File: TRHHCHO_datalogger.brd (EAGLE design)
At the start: 49.1 x 50.8 mm, 39 parts, among them J6 AMP FCI 10103594-0001LF, U1 ATMEGA328P-MU, U10 TSL2591, U2 FT231XQ-R, U3 DS3234, U7 SHT31/35, U8 MCP1703/3.3V, Y2 SPARKFUN_RESONATORSMD

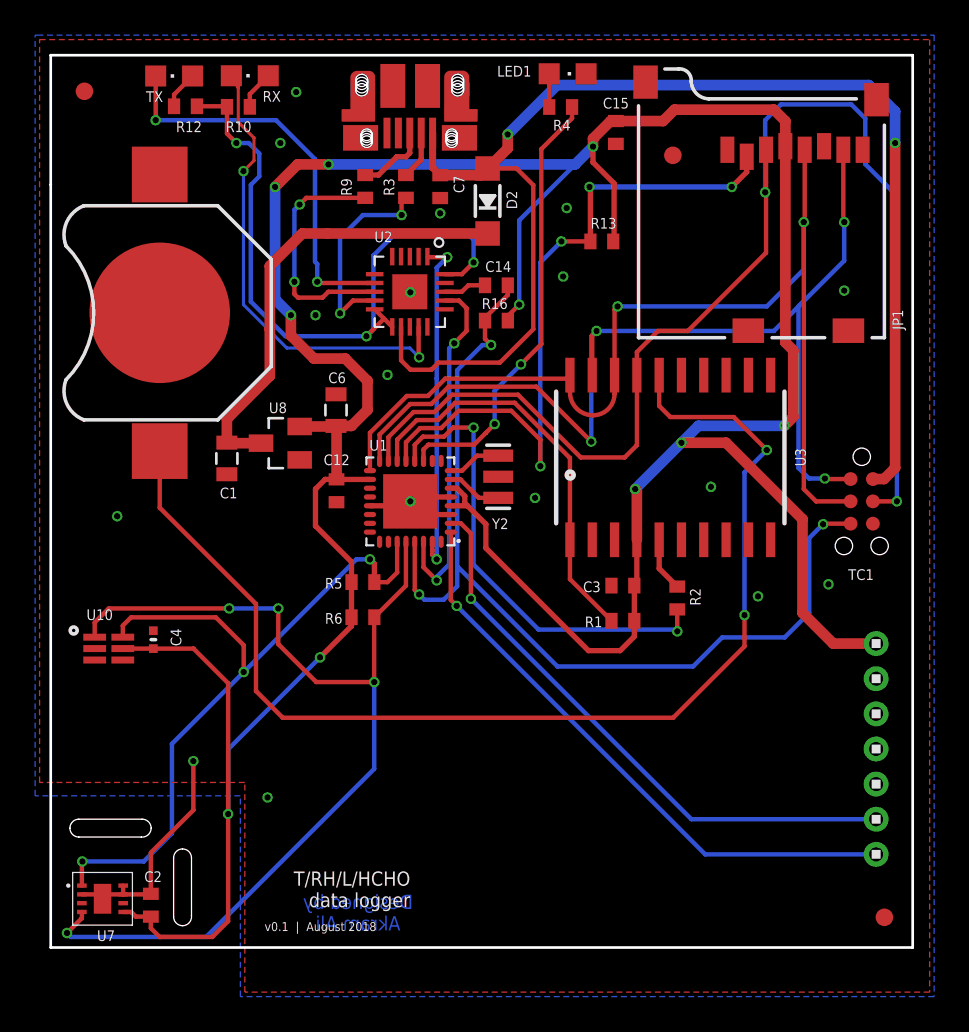
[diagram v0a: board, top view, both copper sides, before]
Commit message: Revert "update"
This reverts commit 3fd739265b7c9a937414b5746fef9af12a5aee94.
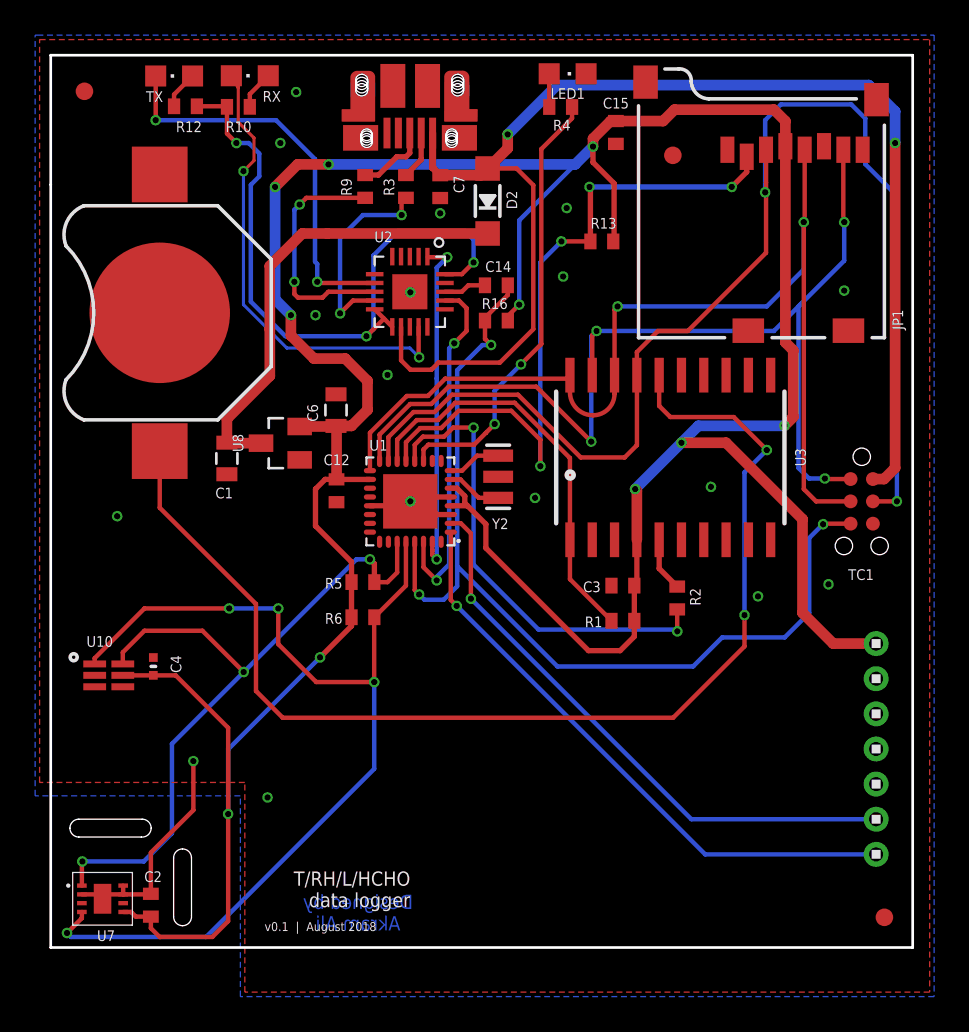
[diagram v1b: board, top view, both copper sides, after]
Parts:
- moved C4 1.52 mm to (14.0, 16.0)
- moved U10 1.52 mm to (11.4, 15.5)
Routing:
- net VCC: track 197.5 -> 195.4 mm
- net SDA: track 42.5 -> 41.6 mm
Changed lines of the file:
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@@
 <element name="LED1" library="adafruit" package="CHIPLED_0805" value="Blue" x="37.5562" y="49.7432" smashed="yes" rot="R270">
 <attribute name="MPN" value="150080BS75000" x="37.5562" y="49.7432" size="1.778" layer="27" rot="R270" display="off"/>
-<attribute name="NAME" x="33.5382" y="49.5832" size="0.6096" layer="25" font="vector"/>
+<attribute name="NAME" x="36.5862" y="48.3132" size="0.6096" layer="25" font="vector"/>
 </element>
 <element name="U8" library="linear" library_urn="urn:adsk.eagle:library:262" package="SOT23" value="MCP1703/3.3V" x="21.1992" y="28.7124" smashed="yes" rot="R90">
 <attribute name="MPN" value="MCP1703T-2502E/CB" x="21.1992" y="28.7124" size="1.778" layer="27" rot="R90" display="off"/>
-<attribute name="NAME" x="21.5766" y="31.0322" size="0.6096" layer="25" font="vector" rot="R180"/>
+<attribute name="NAME" x="19.0942" y="28.2074" size="0.6096" layer="25" font="vector" rot="R90"/>
 </element>
 <element name="C1" library="SparkFun-Capacitors" package="0805" value="1uF" x="18.1558" y="27.8426" smashed="yes" rot="R270">
 <attribute name="MPN" value="CC0805KKX7R7BB105" x="18.1558" y="27.8426" size="1.778" layer="27" rot="R270" display="off"/>
-<attribute name="NAME" x="17.7524" y="25.5703" size="0.6096" layer="25" font="vector"/>
+<attribute name="NAME" x="17.4984" y="25.5703" size="0.6096" layer="25" font="vector"/>
 </element>
 <element name="C6" library="SparkFun-Capacitors" package="0805" value="1uF" x="24.3674" y="30.5942" smashed="yes" rot="R90">
 <attribute name="MPN" value="CC0805KKX7R7BB105" x="24.3674" y="30.5942" size="1.778" layer="27" rot="R90" display="off"/>
-<attribute name="NAME" x="24.9318" y="32.7399" size="0.6096" layer="25" font="vector" rot="R180"/>
+<attribute name="NAME" x="23.3419" y="29.9322" size="0.6096" layer="25" font="vector" rot="R90"/>
 </element>
 <element name="RX" library="adafruit" package="CHIPLED_0805" value="Yellow" x="19.4596" y="49.6314" smashed="yes" rot="R90">
@@
 </element>
 <element name="U$4" library="headers(2mm)" package="1X7" value="1X7" x="55.118" y="11.303" rot="R90"/>
-<element name="U10" library="TSL2591" package="DFN6_TAOS" value="TSL2591" x="11.43" y="17.018" smashed="yes">
-<attribute name="MPN" value="TSL25911FN " x="11.43" y="17.018" size="1.778" layer="27" display="off"/>
-<attribute name="NAME" x="10.16" y="18.642" size="0.6096" layer="25" font="vector"/>
-</element>
-<element name="C4" library="Adafruit Feather 32u4 Bluefruit LE" package="MICROBUILDER__0402MP" value="0.1uF" x="13.97" y="17.526" smashed="yes" rot="R270">
-<attribute name="MPN" value="GRM155R71C104KA88J" x="13.97" y="17.526" size="1.778" layer="27" rot="R270" display="off"/>
-<attribute name="NAME" x="14.9543" y="18.161" size="0.6096" layer="25" font="vector" rot="R270"/>
+<element name="U10" library="TSL2591" package="DFN6_TAOS" value="TSL2591" x="11.43" y="15.494" smashed="yes">
+<attribute name="MPN" value="TSL25911FN " x="11.43" y="15.494" size="1.778" layer="27" display="off"/>
+<attribute name="NAME" x="10.16" y="17.118" size="0.6096" layer="25" font="vector"/>
+</element>
+<element name="C4" library="Adafruit Feather 32u4 Bluefruit LE" package="MICROBUILDER__0402MP" value="0.1uF" x="13.97" y="16.002" smashed="yes" rot="R270">
+<attribute name="MPN" value="GRM155R71C104KA88J" x="13.97" y="16.002" size="1.778" layer="27" rot="R270" display="off"/>
+<attribute name="NAME" x="14.9543" y="16.637" size="0.6096" layer="25" font="vector" rot="R270"/>
 </element>
 </elements>
@@
 <contactref element="C4" pad="2"/>
 <contactref element="U10" pad="5"/>
-<wire x1="12.23" y1="17.018" x2="13.97" y2="17.018" width="0.254" layer="1"/>
-<wire x1="18.228" y1="15.046" x2="16.256" y2="17.018" width="0.254" layer="1"/>
-<wire x1="18.228" y1="7.6" x2="18.228" y2="15.046" width="0.254" layer="1"/>
+<wire x1="12.23" y1="15.494" x2="13.97" y2="15.494" width="0.254" layer="1"/>
+<wire x1="13.97" y1="15.494" x2="15.24" y2="15.494" width="0.254" layer="1"/>
+<wire x1="18.228" y1="12.506" x2="15.24" y2="15.494" width="0.254" layer="1"/>
+<wire x1="18.228" y1="7.6" x2="18.228" y2="12.506" width="0.254" layer="1"/>
 <wire x1="25.252" y1="18.308" x2="25.252" y2="18.8032" width="0.3048" layer="1"/>
-<wire x1="16.256" y1="17.018" x2="13.97" y2="17.018" width="0.254" layer="1"/>
 </signal>
 <signal name="SCL">
@@
 <wire x1="26.543" y1="18.7942" x2="26.552" y2="18.8032" width="0.254" layer="1"/>
 <contactref element="U10" pad="1"/>
-<wire x1="10.63" y1="17.668" x2="10.63" y2="18.504" width="0.254" layer="1"/>
-<wire x1="10.63" y1="18.504" x2="11.43" y2="19.304" width="0.254" layer="1"/>
-<wire x1="11.43" y1="19.304" x2="18.288" y2="19.304" width="0.254" layer="1"/>
+<wire x1="10.63" y1="16.144" x2="10.63" y2="16.472" width="0.254" layer="1"/>
+<wire x1="10.63" y1="16.472" x2="13.462" y2="19.304" width="0.254" layer="1"/>
+<wire x1="13.462" y1="19.304" x2="18.288" y2="19.304" width="0.254" layer="1"/>
 <via x="18.288" y="19.304" extent="1-16" drill="0.35"/>
 <wire x1="18.288" y1="19.304" x2="21.082" y2="19.304" width="0.254" layer="16"/>
@@
 <contactref element="U10" pad="6"/>
 <wire x1="19.1135" y1="15.6845" x2="15.028" y2="11.599" width="0.254" layer="16"/>
-<wire x1="12.23" y1="17.668" x2="12.23" y2="18.326" width="0.254" layer="1"/>
-<wire x1="12.23" y1="18.326" x2="12.7" y2="18.796" width="0.254" layer="1"/>
-<wire x1="12.7" y1="18.796" x2="17.526" y2="18.796" width="0.254" layer="1"/>
-<wire x1="17.526" y1="18.796" x2="19.1135" y2="17.2085" width="0.254" layer="1"/>
+<wire x1="12.23" y1="16.144" x2="12.23" y2="16.802" width="0.254" layer="1"/>
+<wire x1="12.23" y1="16.802" x2="13.462" y2="18.034" width="0.254" layer="1"/>
+<wire x1="13.462" y1="18.034" x2="16.764" y2="18.034" width="0.254" layer="1"/>
+<wire x1="16.764" y1="18.034" x2="19.1135" y2="15.6845" width="0.254" layer="1"/>
 <via x="19.1135" y="15.6845" extent="1-16" drill="0.35"/>
-<wire x1="19.1135" y1="17.2085" x2="19.1135" y2="15.6845" width="0.254" layer="1"/>
 </signal>
 <signal name="N$4">

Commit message: update
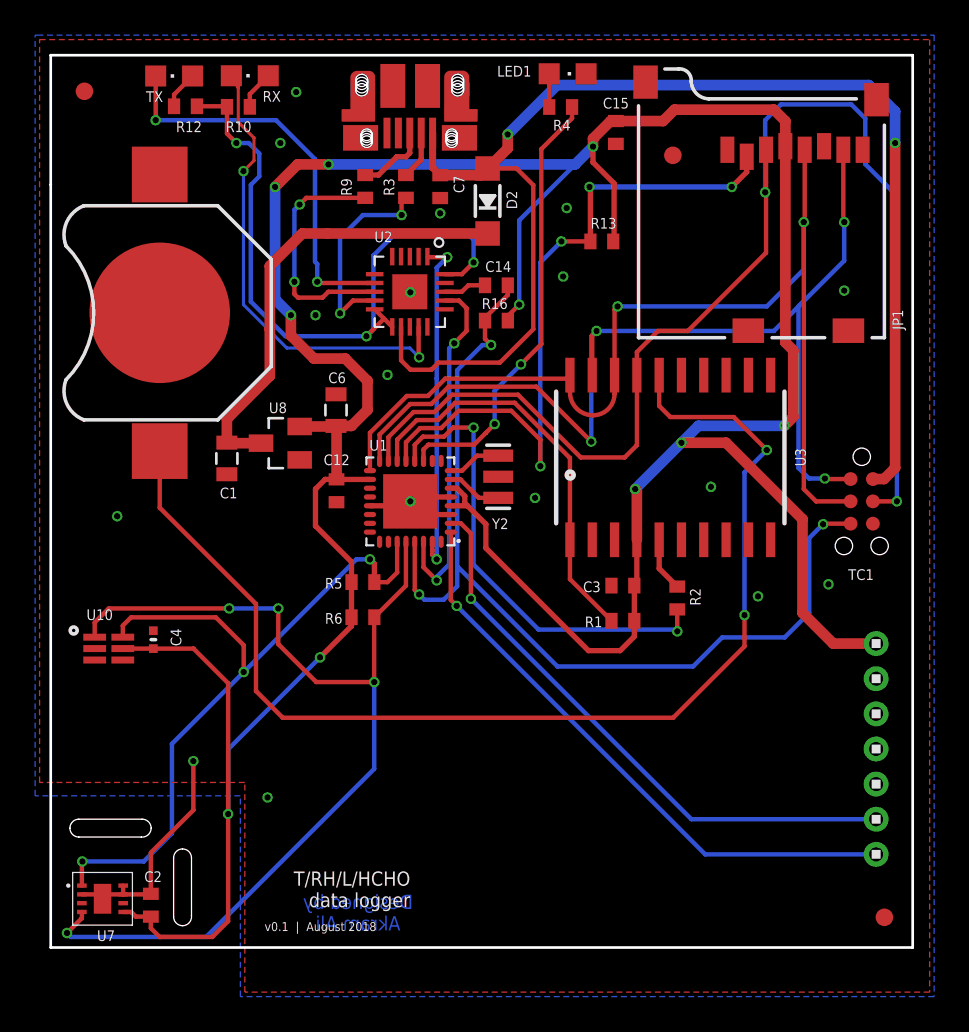
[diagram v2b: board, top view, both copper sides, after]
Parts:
- moved C4 1.52 mm to (14.0, 17.5)
- moved U10 1.52 mm to (11.4, 17.0)
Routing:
- net VCC: track 195.4 -> 197.5 mm
- net SDA: track 41.6 -> 42.5 mm
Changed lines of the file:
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@@
 <element name="LED1" library="adafruit" package="CHIPLED_0805" value="Blue" x="37.5562" y="49.7432" smashed="yes" rot="R270">
 <attribute name="MPN" value="150080BS75000" x="37.5562" y="49.7432" size="1.778" layer="27" rot="R270" display="off"/>
-<attribute name="NAME" x="36.5862" y="48.3132" size="0.6096" layer="25" font="vector"/>
+<attribute name="NAME" x="33.5382" y="49.5832" size="0.6096" layer="25" font="vector"/>
 </element>
 <element name="U8" library="linear" library_urn="urn:adsk.eagle:library:262" package="SOT23" value="MCP1703/3.3V" x="21.1992" y="28.7124" smashed="yes" rot="R90">
 <attribute name="MPN" value="MCP1703T-2502E/CB" x="21.1992" y="28.7124" size="1.778" layer="27" rot="R90" display="off"/>
-<attribute name="NAME" x="19.0942" y="28.2074" size="0.6096" layer="25" font="vector" rot="R90"/>
+<attribute name="NAME" x="21.5766" y="31.0322" size="0.6096" layer="25" font="vector" rot="R180"/>
 </element>
 <element name="C1" library="SparkFun-Capacitors" package="0805" value="1uF" x="18.1558" y="27.8426" smashed="yes" rot="R270">
 <attribute name="MPN" value="CC0805KKX7R7BB105" x="18.1558" y="27.8426" size="1.778" layer="27" rot="R270" display="off"/>
-<attribute name="NAME" x="17.4984" y="25.5703" size="0.6096" layer="25" font="vector"/>
+<attribute name="NAME" x="17.7524" y="25.5703" size="0.6096" layer="25" font="vector"/>
 </element>
 <element name="C6" library="SparkFun-Capacitors" package="0805" value="1uF" x="24.3674" y="30.5942" smashed="yes" rot="R90">
 <attribute name="MPN" value="CC0805KKX7R7BB105" x="24.3674" y="30.5942" size="1.778" layer="27" rot="R90" display="off"/>
-<attribute name="NAME" x="23.3419" y="29.9322" size="0.6096" layer="25" font="vector" rot="R90"/>
+<attribute name="NAME" x="24.9318" y="32.7399" size="0.6096" layer="25" font="vector" rot="R180"/>
 </element>
 <element name="RX" library="adafruit" package="CHIPLED_0805" value="Yellow" x="19.4596" y="49.6314" smashed="yes" rot="R90">
@@
 </element>
 <element name="U$4" library="headers(2mm)" package="1X7" value="1X7" x="55.118" y="11.303" rot="R90"/>
-<element name="U10" library="TSL2591" package="DFN6_TAOS" value="TSL2591" x="11.43" y="15.494" smashed="yes">
-<attribute name="MPN" value="TSL25911FN " x="11.43" y="15.494" size="1.778" layer="27" display="off"/>
-<attribute name="NAME" x="10.16" y="17.118" size="0.6096" layer="25" font="vector"/>
-</element>
-<element name="C4" library="Adafruit Feather 32u4 Bluefruit LE" package="MICROBUILDER__0402MP" value="0.1uF" x="13.97" y="16.002" smashed="yes" rot="R270">
-<attribute name="MPN" value="GRM155R71C104KA88J" x="13.97" y="16.002" size="1.778" layer="27" rot="R270" display="off"/>
-<attribute name="NAME" x="14.9543" y="16.637" size="0.6096" layer="25" font="vector" rot="R270"/>
+<element name="U10" library="TSL2591" package="DFN6_TAOS" value="TSL2591" x="11.43" y="17.018" smashed="yes">
+<attribute name="MPN" value="TSL25911FN " x="11.43" y="17.018" size="1.778" layer="27" display="off"/>
+<attribute name="NAME" x="10.16" y="18.642" size="0.6096" layer="25" font="vector"/>
+</element>
+<element name="C4" library="Adafruit Feather 32u4 Bluefruit LE" package="MICROBUILDER__0402MP" value="0.1uF" x="13.97" y="17.526" smashed="yes" rot="R270">
+<attribute name="MPN" value="GRM155R71C104KA88J" x="13.97" y="17.526" size="1.778" layer="27" rot="R270" display="off"/>
+<attribute name="NAME" x="14.9543" y="18.161" size="0.6096" layer="25" font="vector" rot="R270"/>
 </element>
 </elements>
@@
 <contactref element="C4" pad="2"/>
 <contactref element="U10" pad="5"/>
-<wire x1="12.23" y1="15.494" x2="13.97" y2="15.494" width="0.254" layer="1"/>
-<wire x1="13.97" y1="15.494" x2="15.24" y2="15.494" width="0.254" layer="1"/>
-<wire x1="18.228" y1="12.506" x2="15.24" y2="15.494" width="0.254" layer="1"/>
-<wire x1="18.228" y1="7.6" x2="18.228" y2="12.506" width="0.254" layer="1"/>
+<wire x1="12.23" y1="17.018" x2="13.97" y2="17.018" width="0.254" layer="1"/>
+<wire x1="18.228" y1="15.046" x2="16.256" y2="17.018" width="0.254" layer="1"/>
+<wire x1="18.228" y1="7.6" x2="18.228" y2="15.046" width="0.254" layer="1"/>
 <wire x1="25.252" y1="18.308" x2="25.252" y2="18.8032" width="0.3048" layer="1"/>
+<wire x1="16.256" y1="17.018" x2="13.97" y2="17.018" width="0.254" layer="1"/>
 </signal>
 <signal name="SCL">
@@
 <wire x1="26.543" y1="18.7942" x2="26.552" y2="18.8032" width="0.254" layer="1"/>
 <contactref element="U10" pad="1"/>
-<wire x1="10.63" y1="16.144" x2="10.63" y2="16.472" width="0.254" layer="1"/>
-<wire x1="10.63" y1="16.472" x2="13.462" y2="19.304" width="0.254" layer="1"/>
-<wire x1="13.462" y1="19.304" x2="18.288" y2="19.304" width="0.254" layer="1"/>
+<wire x1="10.63" y1="17.668" x2="10.63" y2="18.504" width="0.254" layer="1"/>
+<wire x1="10.63" y1="18.504" x2="11.43" y2="19.304" width="0.254" layer="1"/>
+<wire x1="11.43" y1="19.304" x2="18.288" y2="19.304" width="0.254" layer="1"/>
 <via x="18.288" y="19.304" extent="1-16" drill="0.35"/>
 <wire x1="18.288" y1="19.304" x2="21.082" y2="19.304" width="0.254" layer="16"/>
@@
 <contactref element="U10" pad="6"/>
 <wire x1="19.1135" y1="15.6845" x2="15.028" y2="11.599" width="0.254" layer="16"/>
-<wire x1="12.23" y1="16.144" x2="12.23" y2="16.802" width="0.254" layer="1"/>
-<wire x1="12.23" y1="16.802" x2="13.462" y2="18.034" width="0.254" layer="1"/>
-<wire x1="13.462" y1="18.034" x2="16.764" y2="18.034" width="0.254" layer="1"/>
-<wire x1="16.764" y1="18.034" x2="19.1135" y2="15.6845" width="0.254" layer="1"/>
+<wire x1="12.23" y1="17.668" x2="12.23" y2="18.326" width="0.254" layer="1"/>
+<wire x1="12.23" y1="18.326" x2="12.7" y2="18.796" width="0.254" layer="1"/>
+<wire x1="12.7" y1="18.796" x2="17.526" y2="18.796" width="0.254" layer="1"/>
+<wire x1="17.526" y1="18.796" x2="19.1135" y2="17.2085" width="0.254" layer="1"/>
 <via x="19.1135" y="15.6845" extent="1-16" drill="0.35"/>
+<wire x1="19.1135" y1="17.2085" x2="19.1135" y2="15.6845" width="0.254" layer="1"/>
 </signal>
 <signal name="N$4">
